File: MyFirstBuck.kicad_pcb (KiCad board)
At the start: 2 copper layers, 130.3 x 127 mm, 43 parts, among them J1 Conn_01x01_Pin, J2 Conn_01x01_Pin, J3 Conn_01x01_Pin, J4 Conn_01x01_Pin, J5 Conn_01x01_Pin, Q1 IRF540N, U1 LM358, U2 LAUNCHXL-F28379D, U3 UCC5304DWVR, U4 TMV 0512SHI

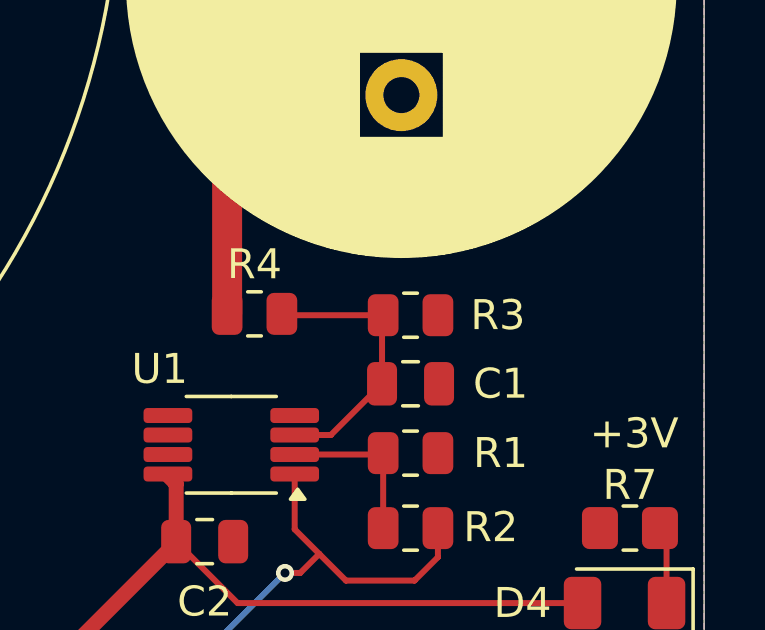
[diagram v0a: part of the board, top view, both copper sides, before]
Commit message: New component changes
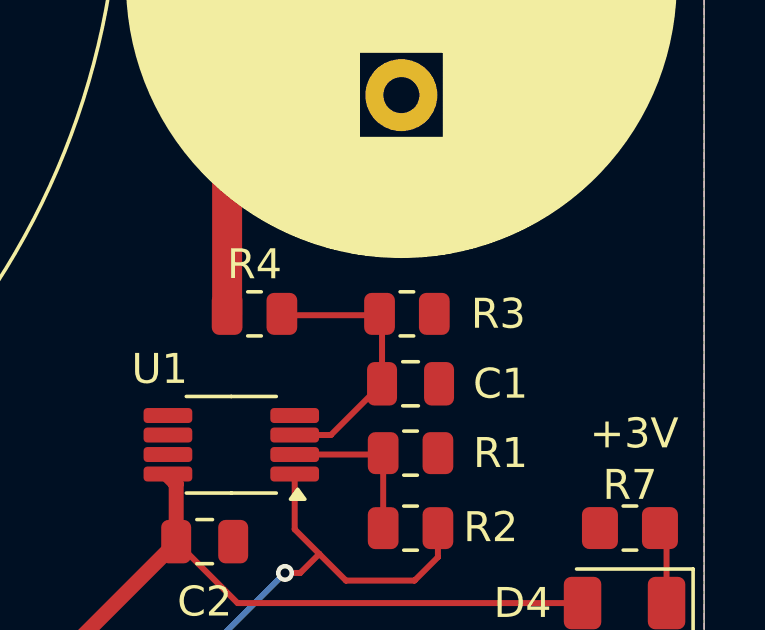
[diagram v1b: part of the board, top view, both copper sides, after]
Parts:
- C1: value 560pF -> 6.8uF
- C2: value C -> 100NF
- R2, R3: value ? -> 600
- moved R3 0.13 mm to (193.3, 82.3), turned to 180 degrees
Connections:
- R3 pad 1: Net-(U1A-+) -> GND
- R3 pad 2: GND -> Net-(U1A-+)
